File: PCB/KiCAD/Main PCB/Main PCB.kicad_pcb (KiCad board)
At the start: 2 copper layers, 120 x 120 mm, 144 parts, among them IC1 ADG608BRZ, IC2 ADG608BRZ, IC3 XB3-24Z8CM, J1 Conn_01x02, J2 Conn_01x02, J3 Conn_01x02, J4 Conn_Coaxial_Small, J5 Conn_01x02, J6 Conn_01x04, J7 Conn_01x04, M1 Conn_01x02_Pin, M2 Conn_01x02_Pin, M3 Conn_01x02_Pin, M4 Conn_01x02_Pin, Q1 BSS138, Q2 BSS138, U2 Teensy4.1, U3 Teensy4.0, U4 LMD18200, U5 LMD18200, U6 LMD18200, U7 LMD18200, U8 MIC5219-3.3YM5

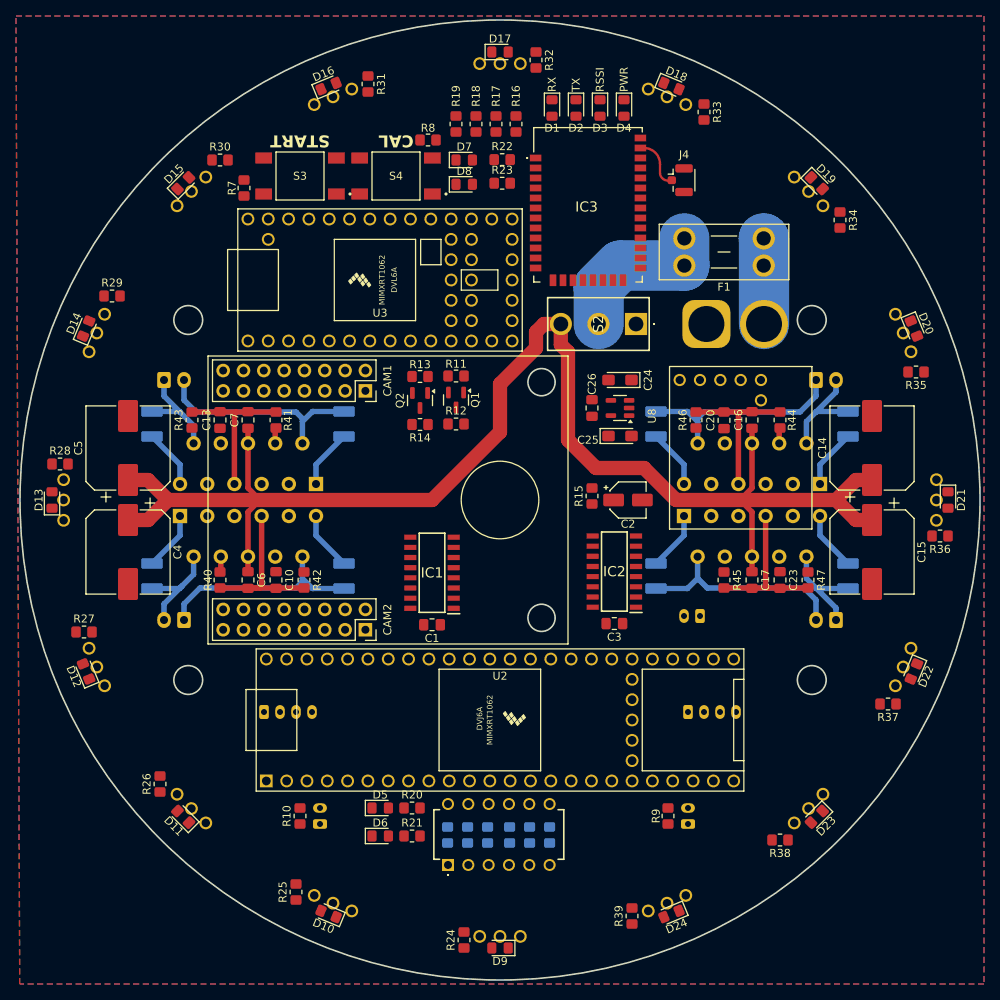
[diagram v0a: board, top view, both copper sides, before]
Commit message: Updated to main PCB
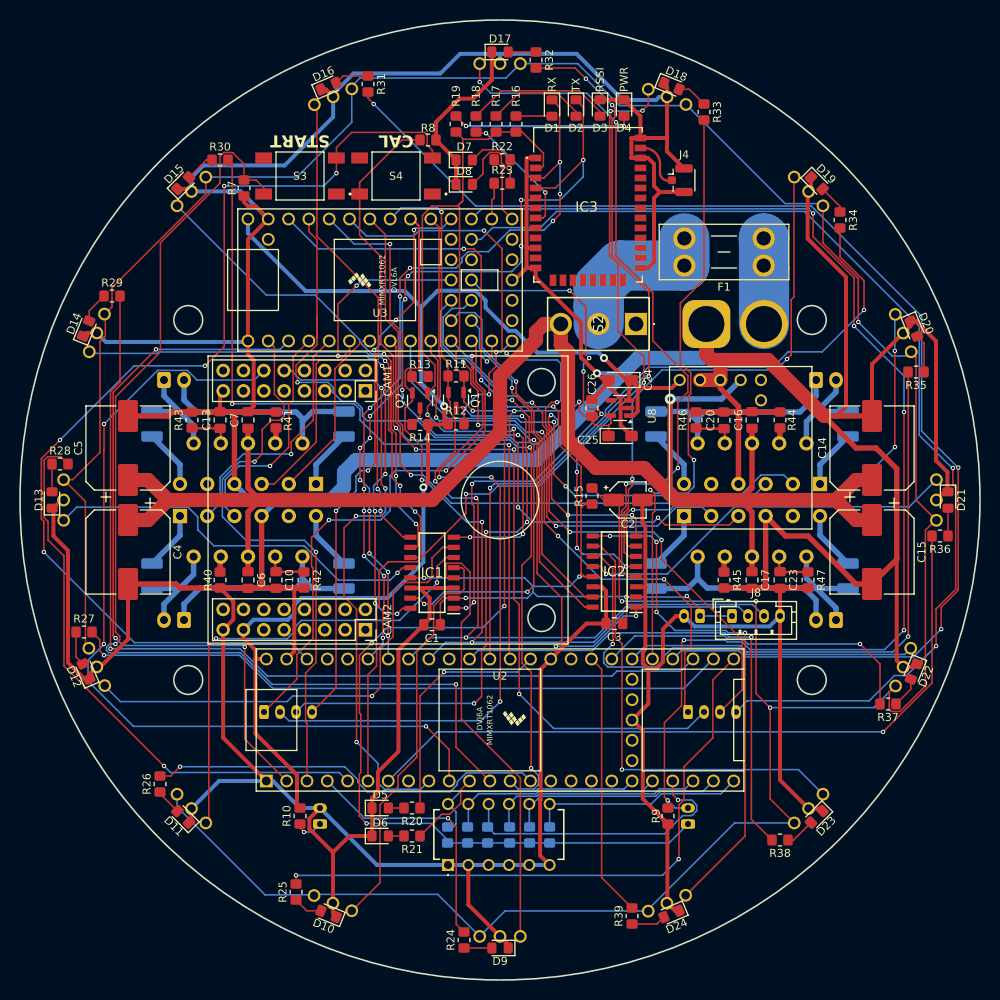
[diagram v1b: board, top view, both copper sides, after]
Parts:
- added J8: Conn_01x04, Connector_JST:JST_PH_B4B-PH-K_1x04_P2.00mm_Vertical, F.Cu at (29.0, 14.5)
- turned D10 to 158 degrees
- turned D12 to 113 degrees
- turned D14 to 68 degrees
- turned D16 to 23 degrees
- turned D18 to -22 degrees
- turned D20 to -67 degrees
- turned D22 to -112 degrees
- turned D24 to -157 degrees
- turned IR10 to -22 degrees
- turned IR12 to -67 degrees
- turned IR14 to -112 degrees
- turned IR16 to -157 degrees
- turned IR2 to 158 degrees
- turned IR4 to 113 degrees
- turned IR6 to 68 degrees
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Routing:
- net GND: track 77.1 -> 964.7 mm, vias 0 -> 1
- net TSSP_PWR: track 0.00 -> 410.8 mm, vias 0 -> 4
- net +3V3: track 0.00 -> 215.3 mm, vias 0 -> 6
- net +5V: track 0.00 -> 163.3 mm, vias 0 -> 3
- net IR_DIR_157.5: track 0.00 -> 158.9 mm, vias 0 -> 3
- net LG_RECEIVE: track 0.00 -> 154.4 mm, vias 0 -> 6
- net +3V3_4_0: track 0.00 -> 147.1 mm, vias 0 -> 8
- net START_BUTTON: track 0.00 -> 137.2 mm, vias 0 -> 2
- net LED_2_A2: track 0.00 -> 134.7 mm, vias 0 -> 2
- net +3V3_4_1: track 0.00 -> 132.3 mm, vias 0 -> 5
- net 3V3_SDA: track 0.00 -> 125.4 mm, vias 0 -> 3
- net IR_DIR_180: track 0.00 -> 119.8 mm, vias 0 -> 4
- net IR_DIR_112.5: track 0.00 -> 119.7 mm, vias 0 -> 1
- net 3V3_SCL: track 0.00 -> 114.6 mm, vias 0 -> 4
- net CAMERA_TX: track 0.00 -> 109.3 mm, vias 0 -> 3
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- removed copper zone on B.Cu, net GND
- removed copper zone on F.Cu, net GND
